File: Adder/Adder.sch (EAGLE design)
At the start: 36 parts, among them IC1 LF356N, IC12 LF356N

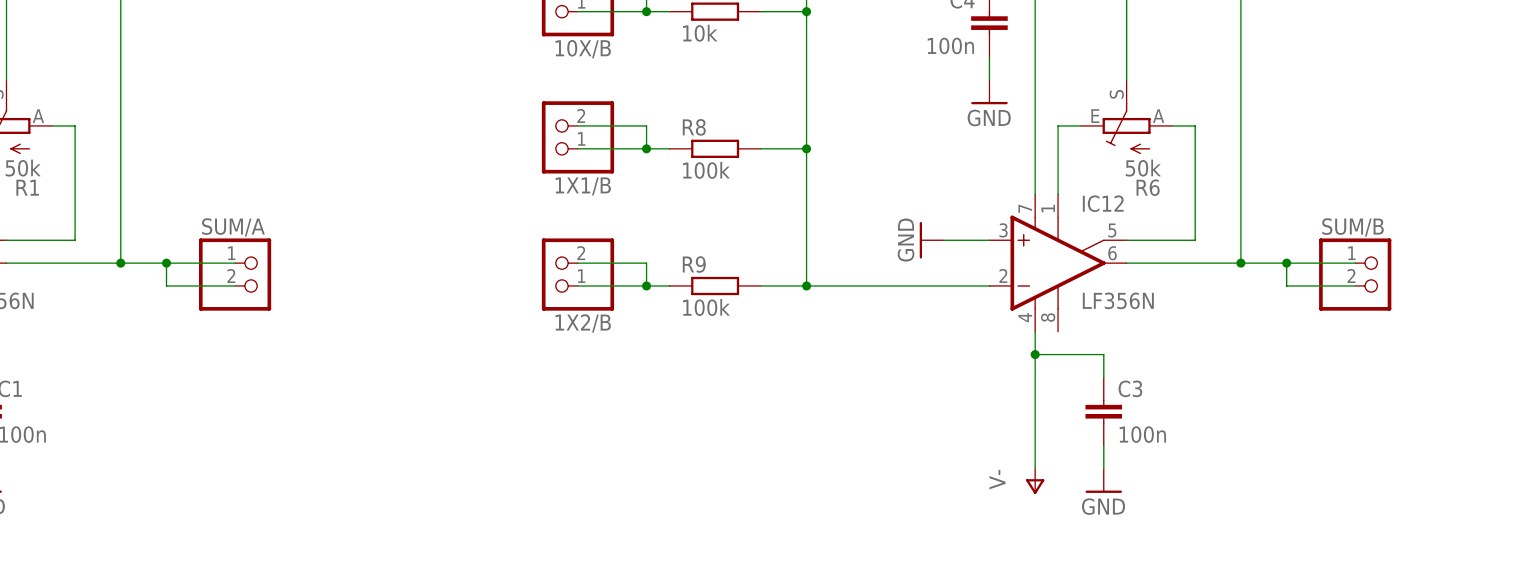
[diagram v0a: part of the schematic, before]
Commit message: Minor fixes
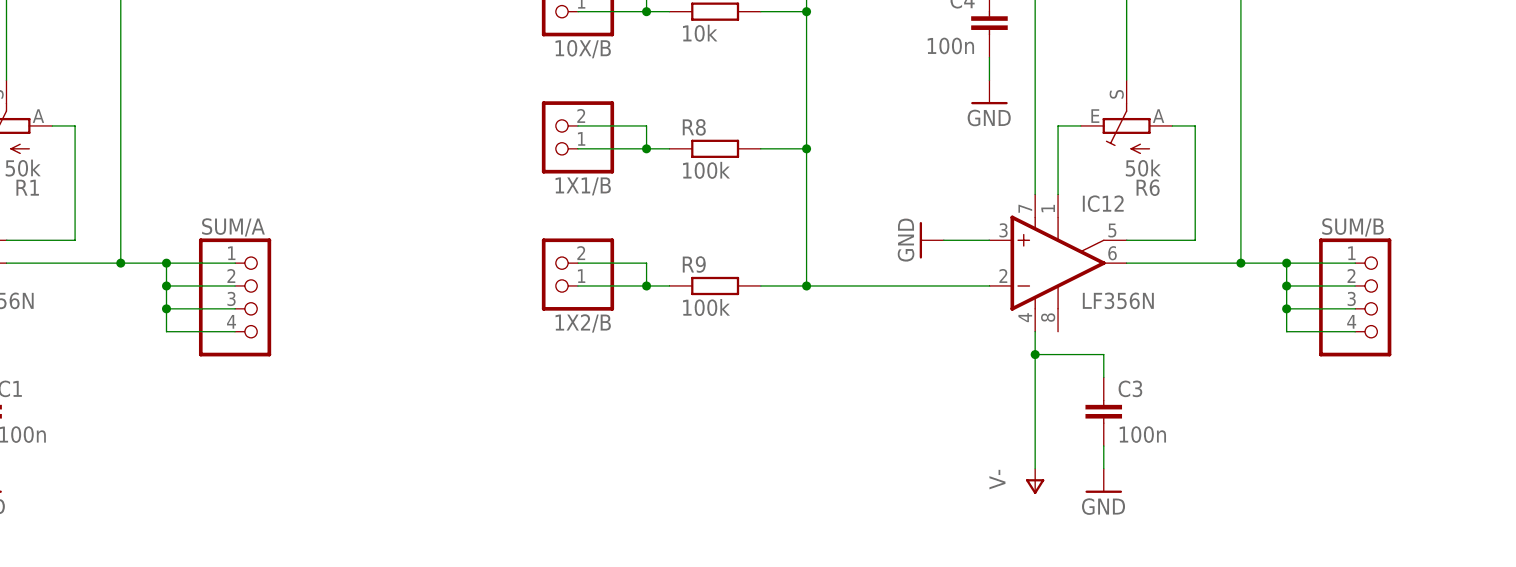
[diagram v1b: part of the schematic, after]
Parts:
- SUM/A, SUM/B: device pinhead:PINHD-1X2 -> pinhead:PINHD-1X4
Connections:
- net N$10: now also SUM/B.3, SUM/B.4
- net N$3: now also SUM/A.3, SUM/A.4
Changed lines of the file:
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@@
 <?xml version="1.0" encoding="utf-8"?>
 <!DOCTYPE eagle SYSTEM "eagle.dtd">
-<eagle version="6.4">
+<eagle version="6.5.0">
 <drawing>
 <settings>
@@
 <part name="P+3" library="supply1" deviceset="V+" device=""/>
 <part name="GND4" library="supply1" deviceset="GND" device=""/>
-<part name="SUM/A" library="pinhead" deviceset="PINHD-1X2" device=""/>
+<part name="SUM/A" library="pinhead" deviceset="PINHD-1X4" device=""/>
 <part name="IC1" library="linear" deviceset="LF356" device="N"/>
 <part name="C2" library="rcl" deviceset="C-EU" device="025-025X050" value="100n"/>
@@
 <part name="P+1" library="supply1" deviceset="V+" device=""/>
 <part name="GND1" library="supply1" deviceset="GND" device=""/>
-<part name="SUM/B" library="pinhead" deviceset="PINHD-1X2" device=""/>
+<part name="SUM/B" library="pinhead" deviceset="PINHD-1X4" device=""/>
 <part name="IC12" library="linear" deviceset="LF356" device="N"/>
 <part name="C4" library="rcl" deviceset="C-EU" device="025-025X050" value="100n"/>
@@
 <instance part="P+3" gate="1" x="78.74" y="160.02"/>
 <instance part="GND4" gate="1" x="86.36" y="93.98"/>
-<instance part="SUM/A" gate="G$1" x="116.84" y="116.84"/>
+<instance part="SUM/A" gate="A" x="116.84" y="114.3"/>
 <instance part="IC1" gate="A" x="81.28" y="119.38"/>
 <instance part="C2" gate="G$1" x="73.66" y="147.32" rot="MR0"/>
@@
 <instance part="P+1" gate="1" x="203.2" y="160.02"/>
 <instance part="GND1" gate="1" x="210.82" y="93.98"/>
-<instance part="SUM/B" gate="G$1" x="241.3" y="116.84"/>
+<instance part="SUM/B" gate="A" x="241.3" y="114.3"/>
 <instance part="IC12" gate="A" x="205.74" y="119.38"/>
 <instance part="C4" gate="G$1" x="198.12" y="147.32" rot="MR0"/>
@@
 <junction x="101.6" y="119.38"/>
 <pinref part="IC1" gate="A" pin="OUT"/>
-<pinref part="SUM/A" gate="G$1" pin="1"/>
-<pinref part="SUM/A" gate="G$1" pin="2"/>
+<pinref part="SUM/A" gate="A" pin="1"/>
+<pinref part="SUM/A" gate="A" pin="2"/>
 <pinref part="R5" gate="G$1" pin="2"/>
+<pinref part="SUM/A" gate="A" pin="3"/>
+<wire x1="114.3" y1="114.3" x2="106.68" y2="114.3" width="0.1524" layer="91"/>
+<wire x1="106.68" y1="114.3" x2="106.68" y2="116.84" width="0.1524" layer="91"/>
+<junction x="106.68" y="116.84"/>
+<pinref part="SUM/A" gate="A" pin="4"/>
+<wire x1="114.3" y1="111.76" x2="106.68" y2="111.76" width="0.1524" layer="91"/>
+<wire x1="106.68" y1="111.76" x2="106.68" y2="114.3" width="0.1524" layer="91"/>
+<junction x="106.68" y="114.3"/>
 </segment>
 </net>
@@
 <junction x="226.06" y="119.38"/>
 <pinref part="IC12" gate="A" pin="OUT"/>
-<pinref part="SUM/B" gate="G$1" pin="1"/>
-<pinref part="SUM/B" gate="G$1" pin="2"/>
+<pinref part="SUM/B" gate="A" pin="1"/>
+<pinref part="SUM/B" gate="A" pin="2"/>
 <pinref part="R10" gate="G$1" pin="2"/>
-</segment>
-</net>
+<pinref part="SUM/B" gate="A" pin="3"/>
+<wire x1="238.76" y1="114.3" x2="231.14" y2="114.3" width="0.1524" layer="91"/>
+<wire x1="231.14" y1="114.3" x2="231.14" y2="116.84" width="0.1524" layer="91"/>
+<junction x="231.14" y="116.84"/>
+<pinref part="SUM/B" gate="A" pin="4"/>
+<wire x1="238.76" y1="111.76" x2="231.14" y2="111.76" width="0.1524" layer="91"/>
+<wire x1="231.14" y1="111.76" x2="231.14" y2="114.3" width="0.1524" layer="91"/>
+<junction x="231.14" y="114.3"/>
+</segment>
+</net>
